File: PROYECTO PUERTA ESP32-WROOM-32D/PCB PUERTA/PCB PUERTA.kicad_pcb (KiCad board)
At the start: 2 copper layers, 91.3 x 69.2 mm, 35 parts, among them J1 LIMIT SWITCHES, J2 LLAVE, J3 Screw_Terminal_01x03, J4 Screw_Terminal_01x02, J5 ALIMENTACION, J6 MOTOR, J7 LAMP, K1 FINDER-36.11, K2 FINDER-36.11, Q1 PZT2222A, Q2 PZT2222A, Q3 PZT2222A, Q4 PZT2222A, SW1 SW_DIP_x04, U1 ESP32-DEVKITC

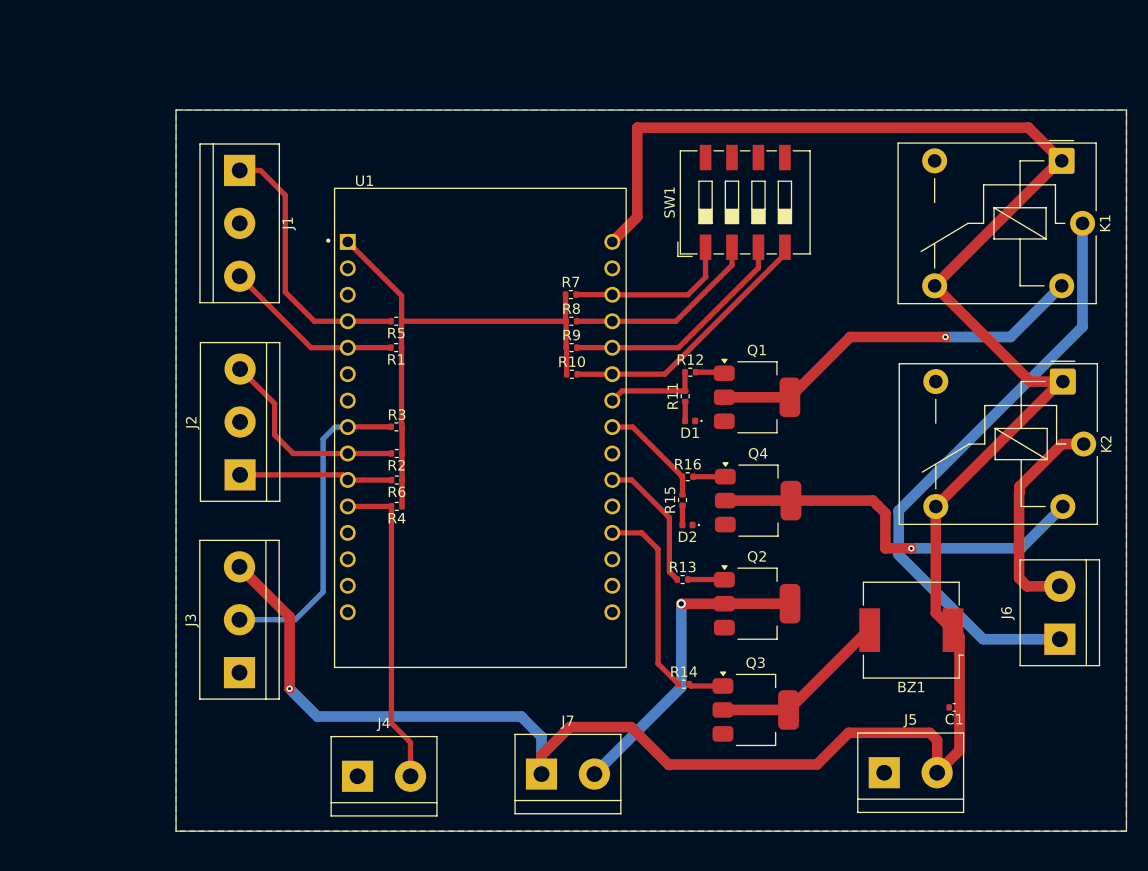
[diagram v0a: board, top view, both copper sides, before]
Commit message: 20.03.2025
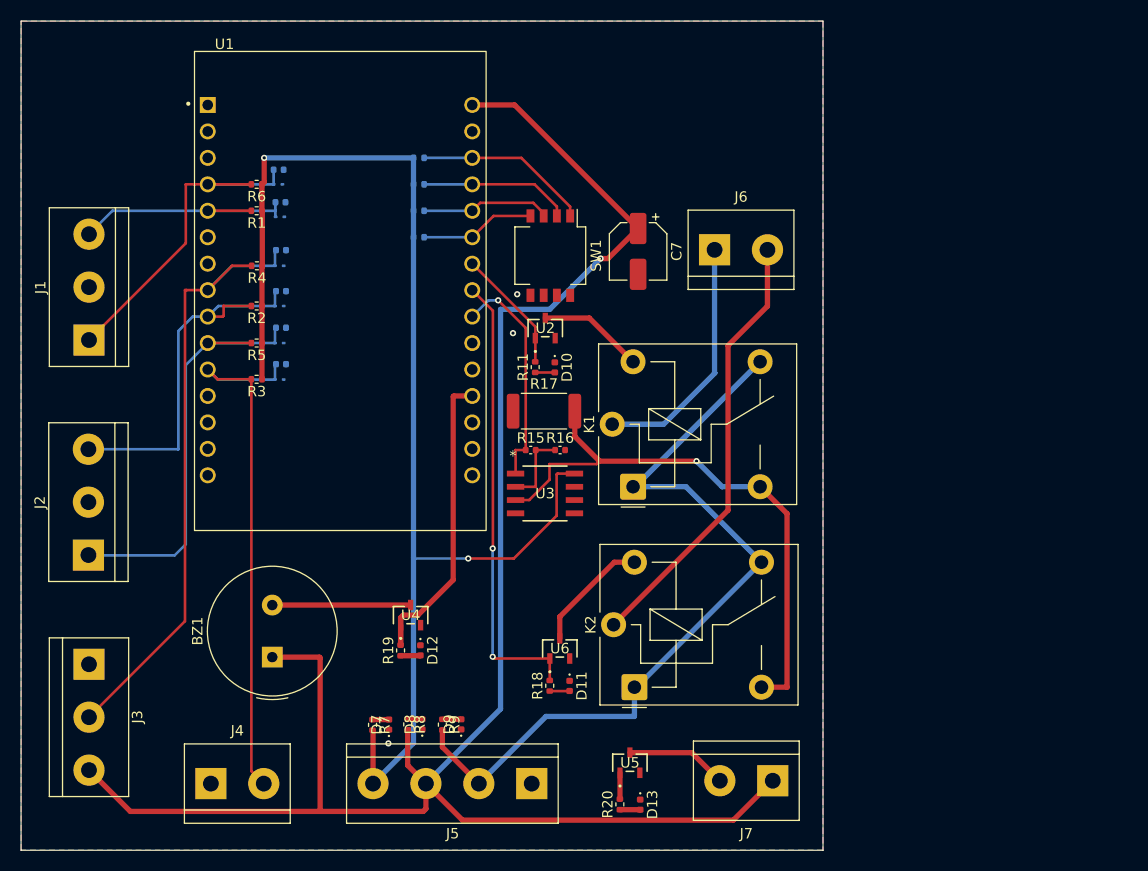
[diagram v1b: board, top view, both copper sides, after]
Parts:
- removed Q1, Q2, Q3, Q4: PZT2222A, Package_TO_SOT_SMD:SOT-223-3_TabPin2
- added C2: 100nF, Capacitor_SMD:C_0402_1005Metric, B.Cu at (110.0, 84.3)
- added C3: 100nF, Capacitor_SMD:C_0402_1005Metric, B.Cu at (110.0, 91.3)
- added C4: 100nF, Capacitor_SMD:C_0402_1005Metric, B.Cu at (110.0, 80.4)
- added C5: 100nF, Capacitor_SMD:C_0402_1005Metric, B.Cu at (110.0, 87.8)
- added C6: 100nF, Capacitor_SMD:C_0402_1005Metric, B.Cu at (109.7, 72.7)
- added C7: 22uF, Capacitor_SMD:CP_Elec_5x5.4, F.Cu at (144.2, 80.5)
- added D10: MA, LED_SMD:LED_0402_1005Metric, F.Cu at (136.2, 91.6)
- added D11: MC, LED_SMD:LED_0402_1005Metric, F.Cu at (137.7, 122.2)
- added D12: MA, LED_SMD:LED_0402_1005Metric, F.Cu at (123.3, 118.8)
- added D13: MA, LED_SMD:LED_0402_1005Metric, F.Cu at (144.4, 133.6)
- added D3: ESD9B3.3ST5G, Diode_SMD:D_SOD-923, B.Cu at (109.8, 92.8)
- added D4: ESD9B3.3ST5G, Diode_SMD:D_SOD-923, B.Cu at (109.8, 81.9)
- added D5: ESD9B3.3ST5G, Diode_SMD:D_SOD-923, B.Cu at (109.8, 89.3)
- added D6: ESD9B3.3ST5G, Diode_SMD:D_SOD-923, B.Cu at (109.7, 74.1)
- added D7: 3V3, LED_SMD:LED_0402_1005Metric, F.Cu at (120.3, 125.9)
- added D8: 5V, LED_SMD:LED_0402_1005Metric, F.Cu at (123.5, 125.9)
- added D9: 12V, LED_SMD:LED_0402_1005Metric, F.Cu at (127.3, 125.9)
- added R17: 0.1, Resistor_SMD:R_2512_6332Metric, F.Cu at (135.2, 95.8)
- added R18: 220, Resistor_SMD:R_0402_1005Metric, F.Cu at (135.8, 122.2)
- added R19: 220, Resistor_SMD:R_0402_1005Metric, F.Cu at (121.4, 118.8)
- added R20: 220, Resistor_SMD:R_0402_1005Metric, F.Cu at (142.5, 133.6)
- added U2: MMUN2233LT1G, LIBRERIA PERSONAL:SOT-23-3_1P4X3P040_ONS-L, F.Cu at (135.3, 87.9)
- added U3: LM358, LIBRERIA PERSONAL:lm358, F.Cu at (135.3, 103.7)
- added U4: MMUN2233LT1G, LIBRERIA PERSONAL:SOT-23-3_1P4X3P040_ONS-L, F.Cu at (122.4, 115.4)
- added U5: MMUN2233LT1G, LIBRERIA PERSONAL:SOT-23-3_1P4X3P040_ONS-L, F.Cu at (143.5, 129.6)
- added U6: MMUN2233LT1G, LIBRERIA PERSONAL:SOT-23-3_1P4X3P040_ONS-L, F.Cu at (136.7, 118.6)
- BZ1: footprint Buzzer_Beeper:Buzzer_CUI_CPT-9019S-SMT -> Buzzer_Beeper:Buzzer_TDK_PS1240P02BT_D12.2mm_H6.5mm
- C1: value 22u -> 100nF; moved to B.Cu
- D1: value MA -> ESD9B3.3ST5G; footprint LED_SMD:LED_0402_1005Metric -> Diode_SMD:D_SOD-923; moved to B.Cu
- D2: value MC -> ESD9B3.3ST5G; footprint LED_SMD:LED_0402_1005Metric -> Diode_SMD:D_SOD-923; moved to B.Cu
- J5: value ALIMENTACION -> Screw_Terminal_01x04; footprint TerminalBlock:TerminalBlock_bornier-2_P5.08mm -> TerminalBlock:TerminalBlock_bornier-4_P5.08mm
- R10, R12, R13, R14: moved to B.Cu
- R15: value 220 -> 100k; footprint Resistor_SMD:R_0402_1005Metric -> Capacitor_SMD:C_0402_1005Metric
- R16: value 1k -> 20k; footprint Resistor_SMD:R_0402_1005Metric -> Capacitor_SMD:C_0402_1005Metric
- R7, R8, R9: value 1k -> 220
- SW1: footprint Button_Switch_SMD:SW_DIP_SPSTx04_Slide_9.78x12.34mm_W8.61mm_P2.54mm -> Button_Switch_SMD:SW_DIP_SPSTx04_Slide_KingTek_DSHP04TS_W7.62mm_P1.27mm
- moved C1 80.9 mm to (109.9, 75.8), turned to 0 degrees
- moved BZ1 61.4 mm to (109.1, 119.5), turned to 90 degrees
- moved K1 51.7 mm to (143.8, 103.1), turned to 90 degrees
- moved K2 50.5 mm to (143.9, 122.3), turned to 90 degrees
- moved J6 50.0 mm to (151.6, 80.3), turned to 0 degrees
- moved R14 49.9 mm to (123.2, 79.1)
- moved R7 45.5 mm to (118.7, 126.0), turned to -90 degrees
- moved D2 44.5 mm to (109.8, 85.7)
- moved D1 44.0 mm to (109.9, 77.2)
- moved R13 43.5 mm to (123.2, 76.6)
- moved R8 41.8 mm to (122.1, 125.9), turned to -90 degrees
- moved R9 38.3 mm to (125.5, 125.9), turned to -90 degrees
- moved J5 33.9 mm to (134.0, 131.6), turned to 180 degrees
- moved R12 31.7 mm to (123.2, 74.1)
- moved R6 31.4 mm to (107.6, 74.1)
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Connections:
- C1 pad 1: +5V -> LSA
- D1 pad 2: Net-(D1-A) -> LSA
- D2 pad 2: Net-(D2-A) -> KEYA
- J5 pad 2: +5V -> +12V
- K1 pad 12: +5V -> +12V
- K1 pad 14: GND -> RefCorriente
- K1 pad A1: +5V -> +12V
- K2 pad 12: +5V -> +12V
- K2 pad 14: GND -> RefCorriente
- K2 pad A1: +5V -> +12V
- R10 pad 2: Net-(U1-D27) -> Net-(U1-D13)
- R11 pad 1: Net-(D1-A) -> Net-(D10-A)
- R12 pad 1: MA -> +3.3V
- R12 pad 2: Net-(Q1-B) -> Net-(U1-D12)
- R13 pad 1: LAMP -> +3.3V
- R13 pad 2: Net-(Q2-B) -> Net-(U1-D14)
- R14 pad 1: BUZZER -> +3.3V
- R14 pad 2: Net-(Q3-B) -> Net-(U1-D27)
- R15 pad 1: Net-(D2-A) -> Net-(U1-D33)
- R15 pad 2: MC -> Net-(U3A--)
- R16 pad 1: MC -> Net-(U3A--)
- R16 pad 2: Net-(Q4-B) -> GND
- R3 pad 2: FTC -> PP
- R4 pad 2: PP -> FTC
- R5 pad 2: LSC -> KEYC
- R6 pad 2: KEYC -> LSC
- R7 pad 1: +3.3V -> Net-(D7-A)
- R7 pad 2: Net-(U1-D13) -> +3.3V
- R8 pad 1: +3.3V -> Net-(D8-A)
- R8 pad 2: Net-(U1-D12) -> +5V
- R9 pad 1: +3.3V -> Net-(D9-A)
- R9 pad 2: Net-(U1-D14) -> +12V
- U1 pad 1: +3.3V -> unconnected-(U1-3V3-Pad1)
- U1 pad 22: unconnected-(U1-D33-Pad22) -> Net-(U1-D33)
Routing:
- net +12V: track 0.00 -> 76.7 mm
- net +3.3V: track 51.1 -> 123.8 mm, vias 0 -> 2
- net RefCorriente: track 0.00 -> 55.5 mm, vias 0 -> 1
- net +5V: track 222.4 -> 183.9 mm
- net MO1: track 58.0 -> 23.7 mm
- net MC: track 10.4 -> 43.7 mm, vias 0 -> 2
- net FTC: track 30.8 -> 61.2 mm
- net KEYC: track 14.7 -> 42.2 mm
- net Net-(U2-COLLECTOR): track 36.8 -> 10.2 mm, vias 1 -> 0
- net Net-(U6-COLLECTOR): track 38.0 -> 11.4 mm, vias 1 -> 0
- net Net-(U1-D33): track 0.00 -> 21.8 mm, vias 0 -> 1
- net PP: track 30.9 -> 52.3 mm
- net MO2: track 20.9 -> 42.1 mm
- net Net-(J7-Pin_2): track 30.2 -> 9.75 mm, vias 1 -> 0
- net KEYA: track 19.7 -> 36.9 mm
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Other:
- board size 91.3 x 69.2 mm -> 77 x 79.6 mm
